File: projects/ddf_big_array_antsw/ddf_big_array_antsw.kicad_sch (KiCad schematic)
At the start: 40 parts, among them J1 Conn_Coaxial, J2 Conn_Coaxial, J3 Conn_Coaxial, J4 Conn_Coaxial, J5 Conn_Coaxial, J6 RJ45_Shielded, J7 5_Port_50Z_RF_Junction

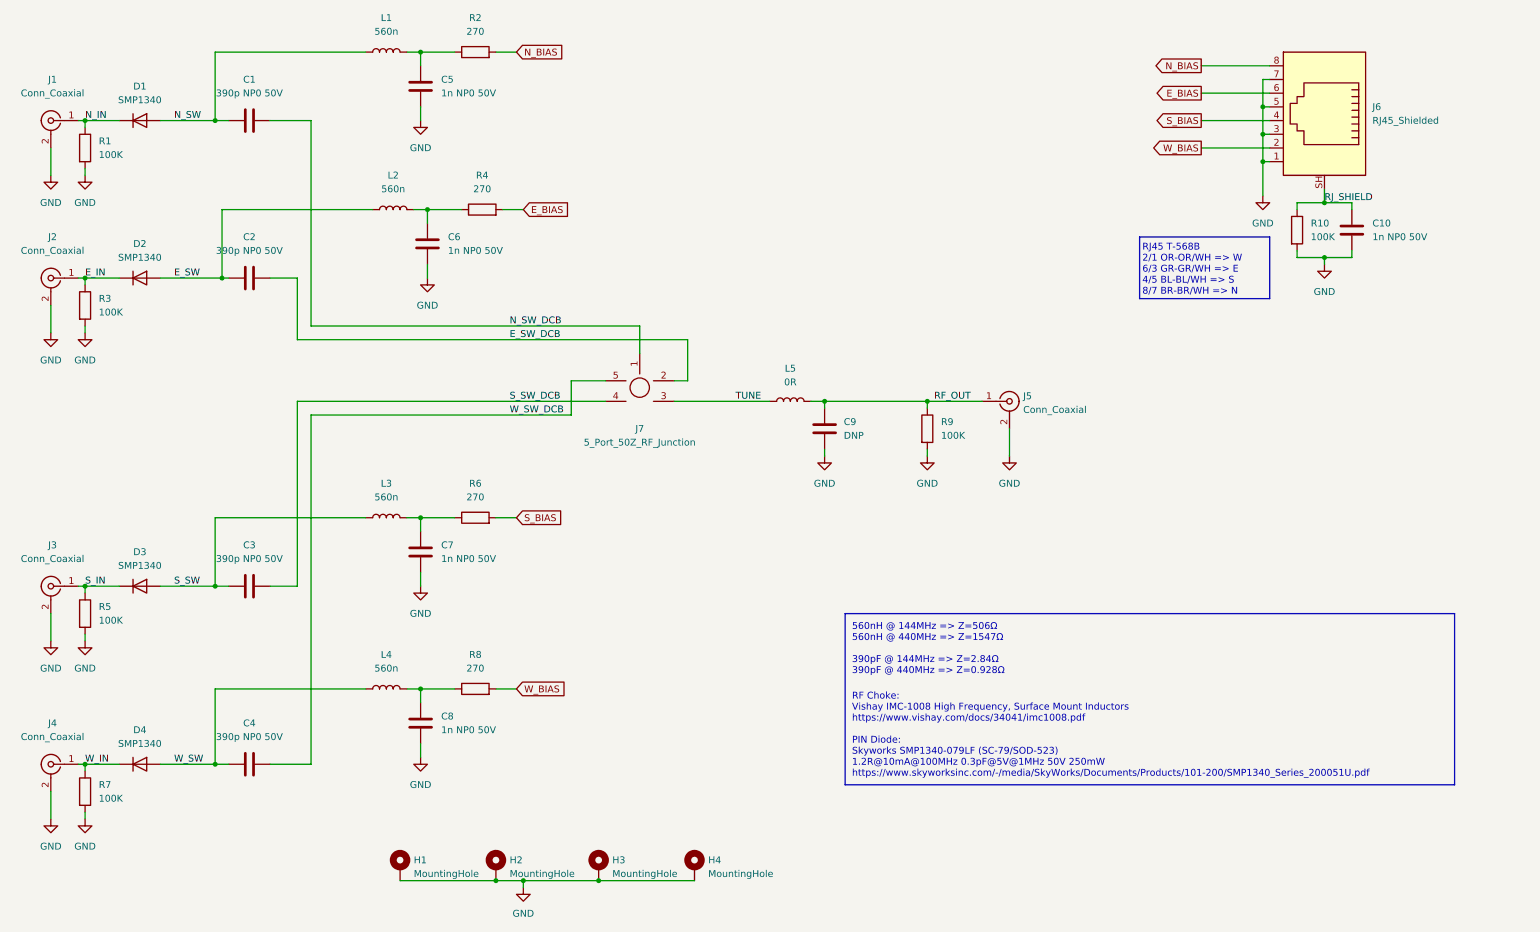
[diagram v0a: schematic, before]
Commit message: release candidate
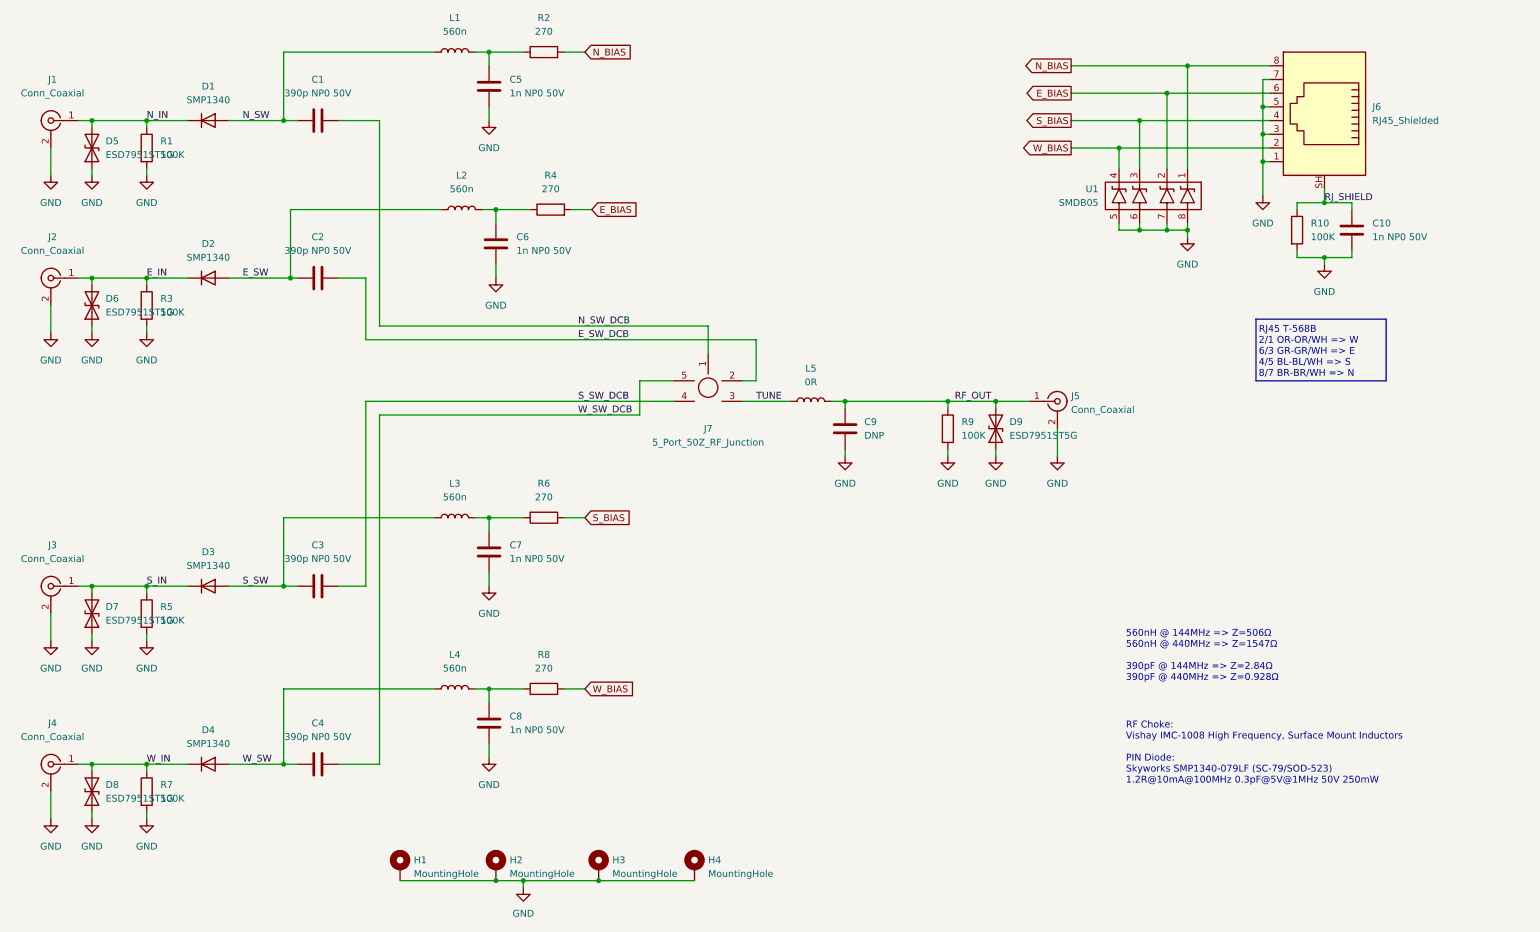
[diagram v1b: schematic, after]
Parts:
- added D5, D6, D7, D8, D9: ESD7951ST5G, Diode_SMD:D_SOD-923, symbol Device:D_TVS
- added U1: SMDB05, Package_SO:SO-8_3.9x4.9mm_P1.27mm, symbol ch:TVS 4x Unidir
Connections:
- net E_BIAS: now also U1.2 (B1)
- net E_IN: now also D6.2 (A2)
- net GND: now also D5.1 (A1), D6.1 (A1), D7.1 (A1), D8.1 (A1), D9.1 (A1), U1.5 (D2), U1.6 (C2), U1.7 (B2), U1.8 (A2)
- net N_BIAS: now also U1.1 (A1)
- net N_IN: now also D5.2 (A2)
- net RF_OUT: now also D9.2 (A2)
- net S_BIAS: now also U1.3 (C1)
- net S_IN: now also D7.2 (A2)
- net W_BIAS: now also U1.4 (D1)
- net W_IN: now also D8.2 (A2)
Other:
- note added: "RF Choke: Vishay IMC-1008 High Frequency, Surface Mount Inductors PIN Diode: Skyworks SMP1340-079LF (SC-79/SOD-523) 1.2R@10mA@100MHz 0.3pF@5V@1MHz 50V 250mW"
- note removed: "RF Choke: Vishay IMC-1008 High Frequency, Surface Mount Inductors https://www.vishay.com/docs/34041/imc1008.pdf PIN Diode: Skyworks SMP1340-079LF (SC-79/SOD-523) 1.2R@10mA@100MHz 0.3pF@5V@1MHz 50V 250mW https://www.skyworksinc.com/-/media/SkyWorks/Documents/Products/101-200/SMP1340_Series_200051U.pdf"
- moved on the sheet: C1, C2, C3, C4, C5, C6, C7, C8, C9, D1, D2, D3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
